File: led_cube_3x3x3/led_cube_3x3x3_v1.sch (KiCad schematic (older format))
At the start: 50 parts, among them IC1 ATMEGA8A-P

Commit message: led cube sch v1
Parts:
- removed ??1: ST2221C, ~, symbol ST2221C
- removed D1, D? (x26): LED, ~, symbol LED
- added C1, C12, C13, C3, C5, C7, C8, C9: 100n, ~, symbol C
- added C10, C11: 33p, ~, symbol C
- added C14, C2, C4, C6: 10u, ~, symbol CP1
- added D1: LED_CUBE_3X3X3, symbol LED_CUBE_3X3X3
- added J1: Supply, symbol CONN_2
- added J2: ISP, AVR-ISP-6, symbol AVR-ISP-6
- added J3: SPI, symbol DIL8
- added L1: 15uH, ~, symbol INDUCTOR_SMALL
- added Q4: SFH320, ~, symbol OPTO_NPN
- added R1, R11, R2, R3: 10k, ~, symbol R
- added R10, R6, R8: 0R, ~, symbol R
- added R30: 20R, SM0805, symbol R
- added R31: 1k1, ~, symbol R
- added R32, R33: 100R, ~, symbol R
- added R34: 2k, ~, symbol R
- added R4: 20R, ~, symbol R
- added R5, R7, R9: 230R, ~, symbol R
- added U1: ST2221C, ~, symbol ST2221C
- added U2: 24C512, symbol 24C512
- added X1: 16MHz, ~, symbol CRYSTAL
- gave numbers to parts that had none: 21
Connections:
- net labels added: +5V, A1, A2, A3, AGND, ARef, AVcc, C1, C2, C3, C4, C5, C6, C7, C8, C9, CLK, GND, ISP MISO, ISP MOSI, ISP RST, ISP SCK, ISP SS, LA, LIGHT_SENS, Lev_1, Lev_2, Lev_3, OE, RxD, SCL, SDA, SDI, SDO, TxD, Vert_1, Vert_2, Vert_3, Vert_4, Vert_5, Vert_6, Vert_7, Vert_8, Vert_9, WP, uCVcc
- wire segments 126 -> 218
- no-connect marks 0 -> 10
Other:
- note added: "150mA"
- note added: "Constant Current\nLED Driver"
- note added: "EEPROM"
- note added: "ISP"
- note added: "LEDs"
- note added: "Light sens"
- note added: "MAX 75mA\nper output"
- note added: "Microcontroller"
- note added: "SPI Connector"
- note added: "Supply\nConnector"
- note removed: "75mA per output max"
- moved on the sheet: IC1, Q1, Q2, Q3, R13, R15, R17, R19, R21, R23, R25, R27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

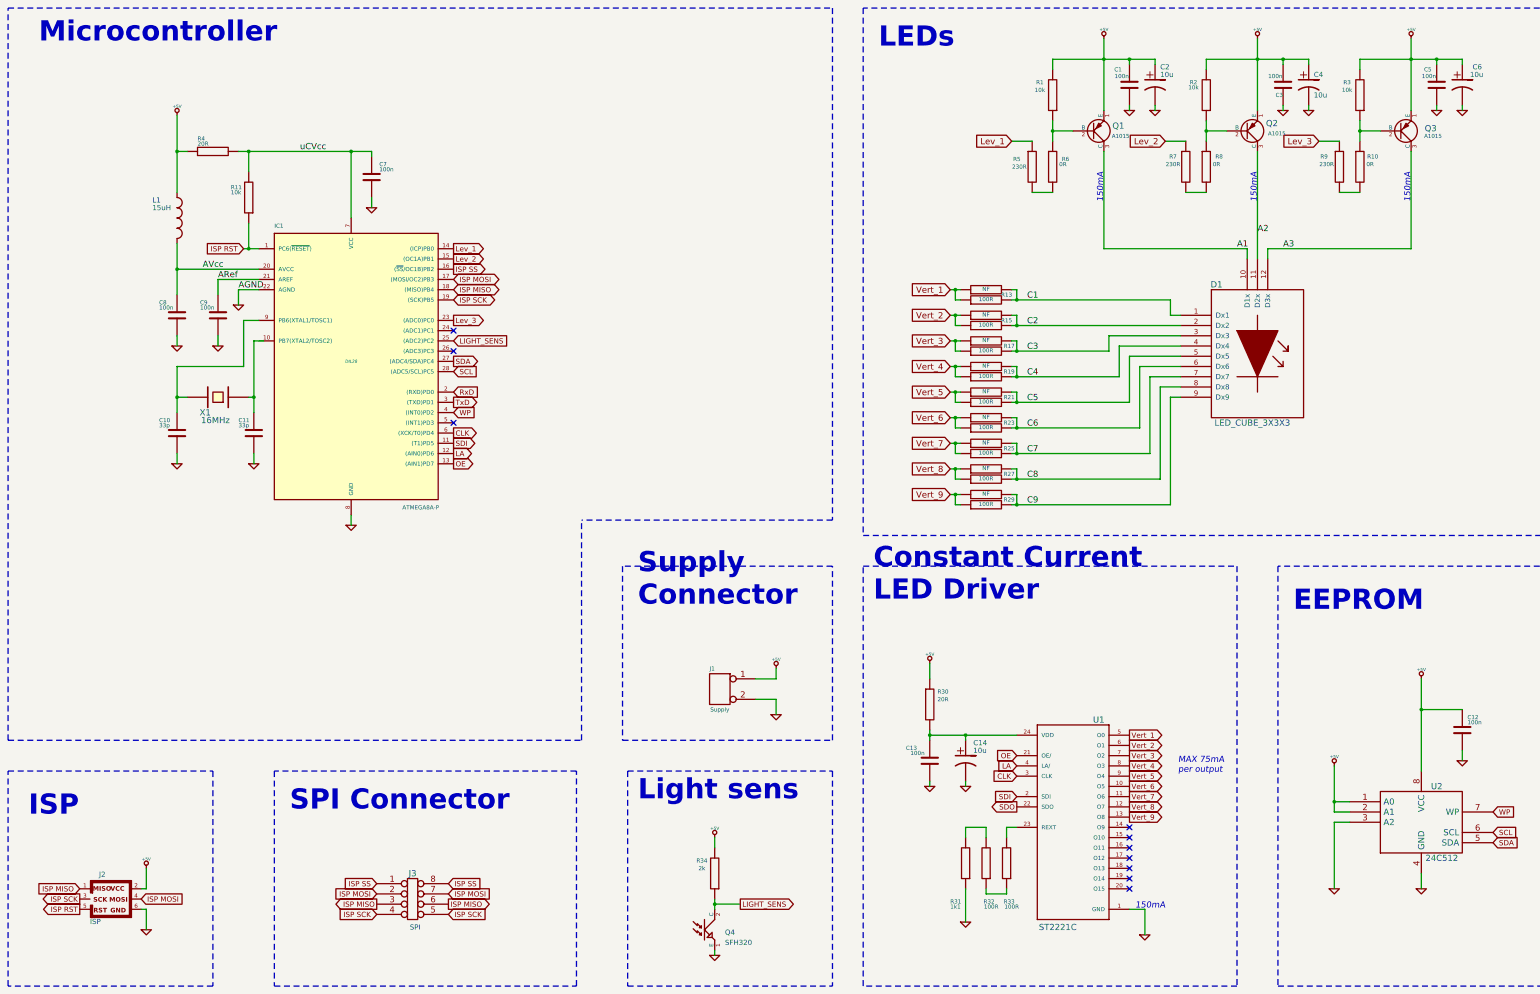
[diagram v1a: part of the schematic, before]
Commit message: led cube pcb v0.1
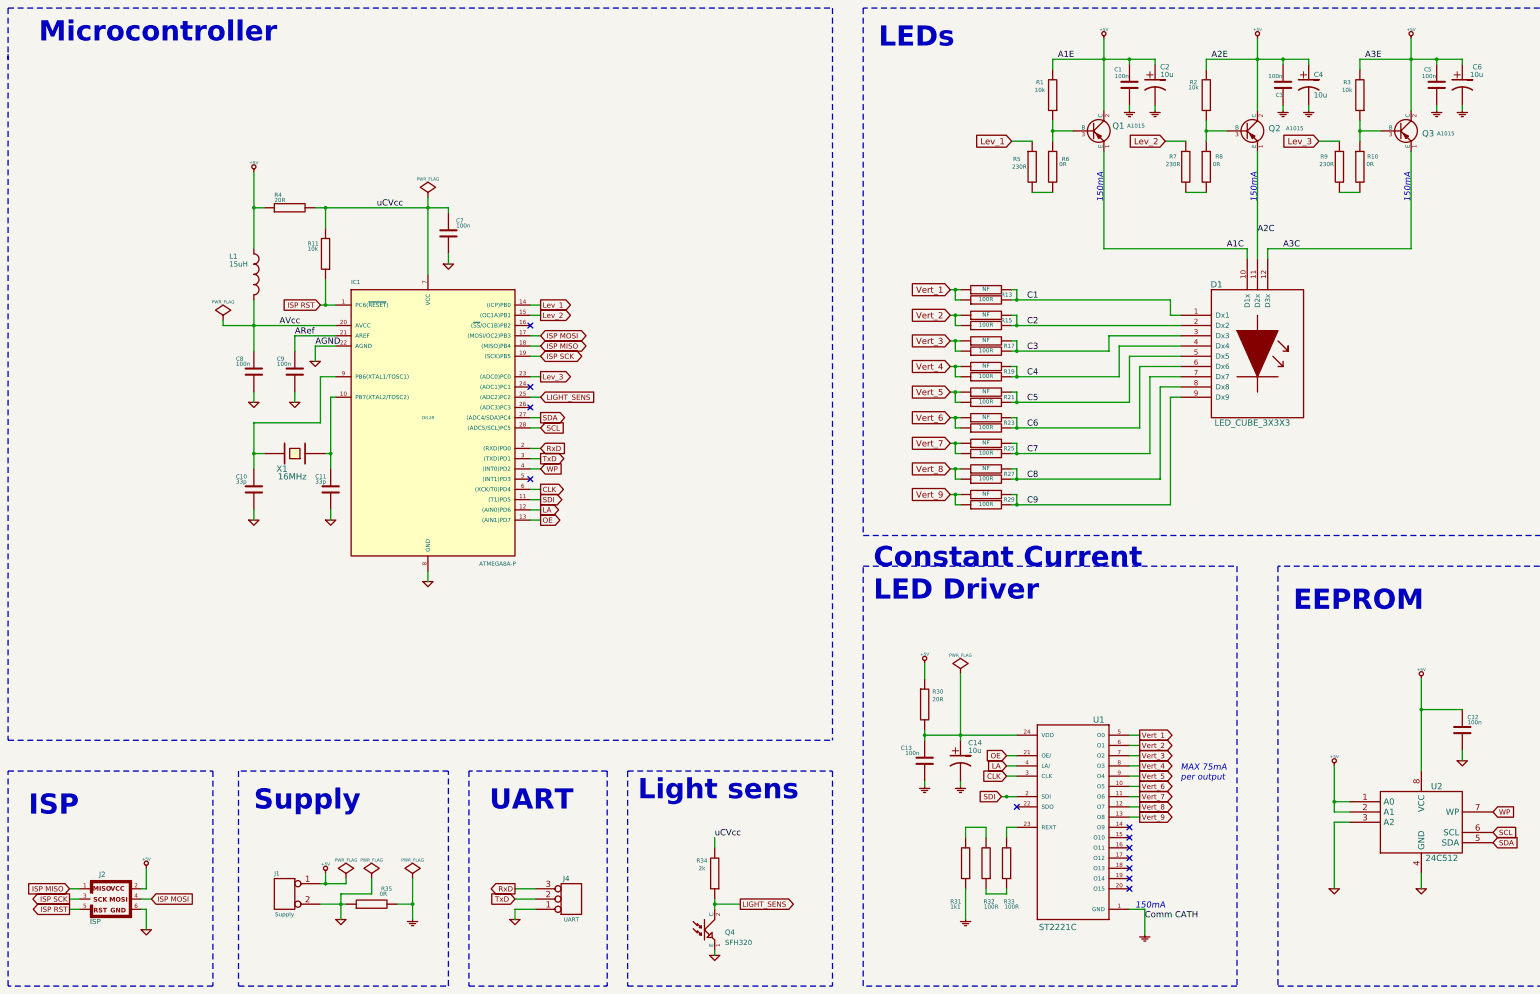
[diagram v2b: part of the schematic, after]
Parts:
- removed J3: SPI, symbol DIL8
- removed Q1, Q2, Q3: A1015, TO92, symbol PNP
- added J4: UART, symbol CONN_3
- added Q1, Q2, Q3: A1015, ~, symbol PNP2
- added R35: 0R, SM0805, symbol R
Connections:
- net +5V: now also Q1.2 (C), Q2.2 (C), Q3.2 (C); no longer R34.2
- net GND: now also J4.1 (P1), R35.1; no longer C1.1, C13.1, C14.2, C2.2, C3.1, C4.2, C5.1, C6.2, R31.1, U1.1 (GND)
- net RxD: now also J4.3 (P3)
- net TxD: now also J4.2 (PM)
- net uCVcc: now also R34.2
- net at IC1.10 (PB7(XTAL2/TOSC2)): now also C11.1, X1.1
- net at R1.1, R6.1: now also Q1.3 (B)
- net at R2.1, R8.1: now also Q2.3 (B)
- net at R10.1, R3.1: now also Q3.3 (B)
- net A1 renamed A1C
- net A1C: now also Q1.1 (E)
- net A2 renamed A2C
- net A2C: now also Q2.1 (E)
- net A3 renamed A3C
- net A3C: now also Q3.1 (E)
- net ISP SS: no longer names the net of IC1.16 ((~SS~/OC1B)PB2)
- net SDO: no longer names the net of U1.22 (SDO)
- new net GNDPWR: C1.1, C13.1, C14.2, C2.2, C3.1, C4.2, C5.1, C6.2, R31.1, R35.2, U1.1 (GND)
- no-connect marks 10 -> 12
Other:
- note added: "Supply"
- note added: "UART"
- note removed: "SPI Connector"
- note removed: "Supply\nConnector"
- moved on the sheet: C10, C11, C13, C14, C7, C8, C9, IC1, J1, L1, R11, R30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
